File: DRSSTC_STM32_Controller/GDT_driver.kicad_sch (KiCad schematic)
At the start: 60 parts, among them IC1 UCC27282DR, IC2 UCC27282DR, IC3 UCC27282DR, IC4 UCC27282DR, IC5 SN74LVC14ADR, IC6 SN74LVC11ADR, IC7 SN74LVC11ADR, Q1 QM6006D, Q15 QM6006D, Q16 QM6006D, Q17 QM6006D, Q18 QM6006D, Q2 QM6006D, Q3 QM6006D, Q4 QM6006D

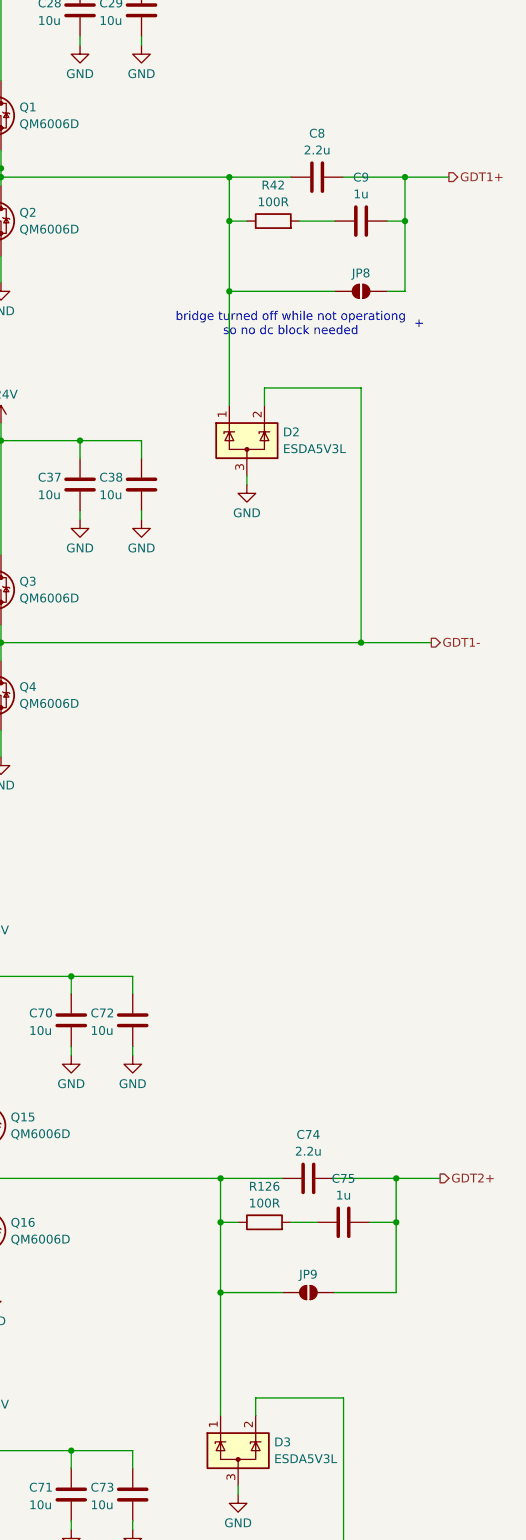
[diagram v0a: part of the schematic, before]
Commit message: start routing
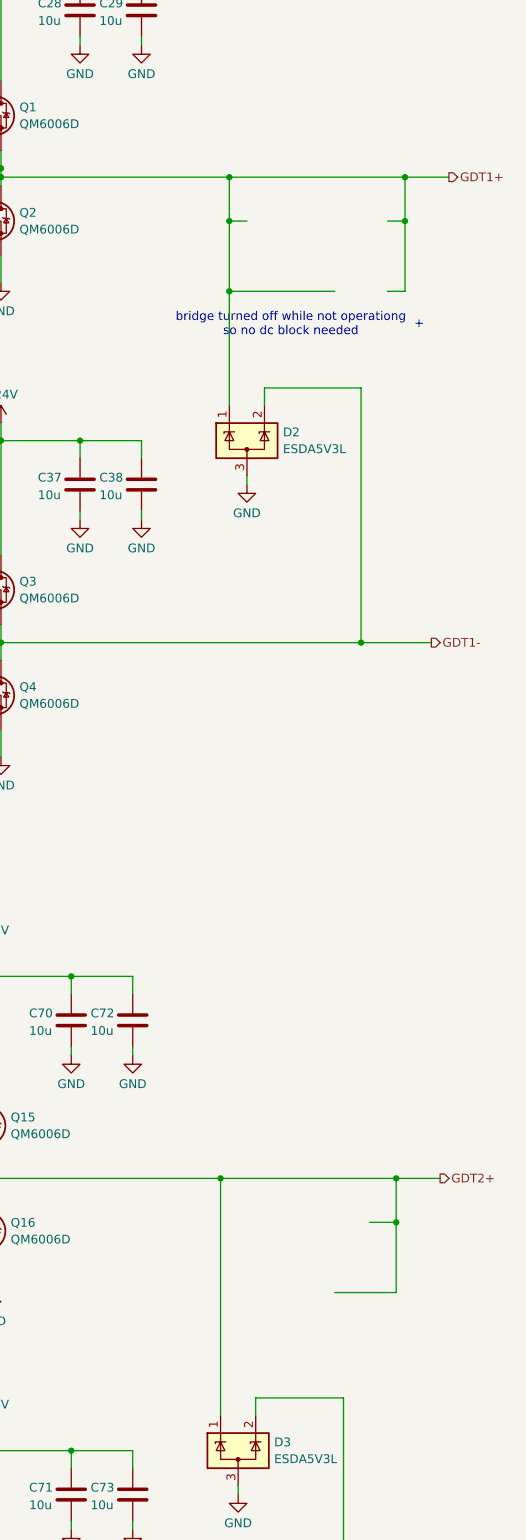
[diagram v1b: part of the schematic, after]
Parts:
- removed C74, C8: 2.2u, Capacitor_THT:C_Axial_L12.0mm_D7.5mm_P15.00mm_Horizontal, symbol Device:C
- removed C75, C9: 1u, Capacitor_THT:C_Axial_L12.0mm_D7.5mm_P15.00mm_Horizontal, symbol Device:C
- removed JP8, JP9: SolderJumper_2_Open, Jumper:SolderJumper-2_P1.3mm_Open_RoundedPad1.0x1.5mm, symbol Jumper:SolderJumper_2_Open
- removed R126, R42: 100R, Resistor_THT:R_Axial_DIN0309_L9.0mm_D3.2mm_P12.70mm_Horizontal, symbol Device:R
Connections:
- net GDT1+: now also C45.2, D2.1 (K), IC1.4 (HS), Q1.3 (S), Q2.2 (D)
- net GDT2+: now also C68.2, D3.1 (K), IC3.4 (HS), Q15.3 (S), Q16.2 (D)
